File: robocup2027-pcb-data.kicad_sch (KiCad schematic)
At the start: 48 parts, among them M5 Motor_Servo, M6 Motor_Servo, Q1 BPW40, Q2 BPW40, U1 ESP32-DEVKITC-32E

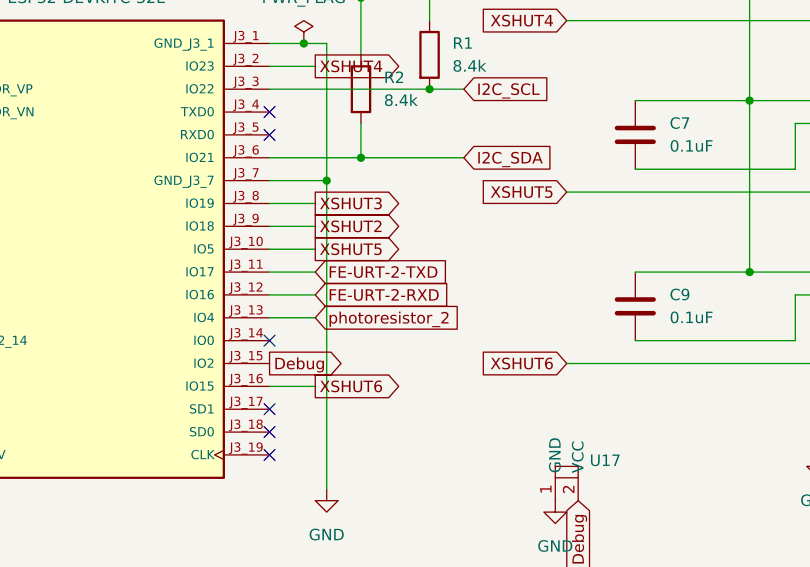
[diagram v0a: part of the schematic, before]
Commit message: fix pim
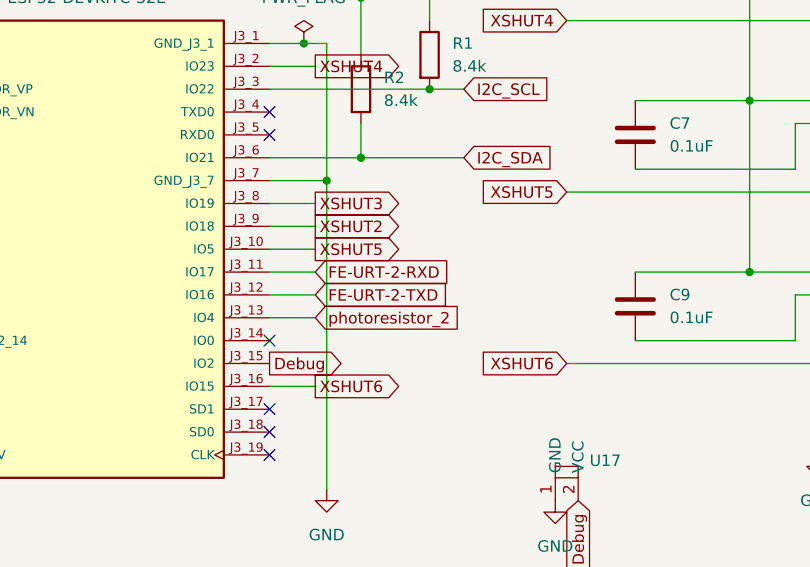
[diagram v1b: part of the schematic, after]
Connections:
- net FE-URT-2-RXD: now also U1.J3_11 (IO17); no longer U1.J3_12 (IO16)
- net FE-URT-2-TXD: now also U1.J3_12 (IO16); no longer U1.J3_11 (IO17)
